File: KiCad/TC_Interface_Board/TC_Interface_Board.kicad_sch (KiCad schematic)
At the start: 23 parts, among them J1_24V_ROW1 Conn_01x04, J1_CN1_24V1 Conn_01x03, J2_CN2_9V_Main1 Conn_01x02, J3_CN3_9V_Main1 Conn_01x02, J4_BUS_MONITER1 Conn_01x05, Q1 DTC143E, Q2 DTC143E, U1 MC34063AP

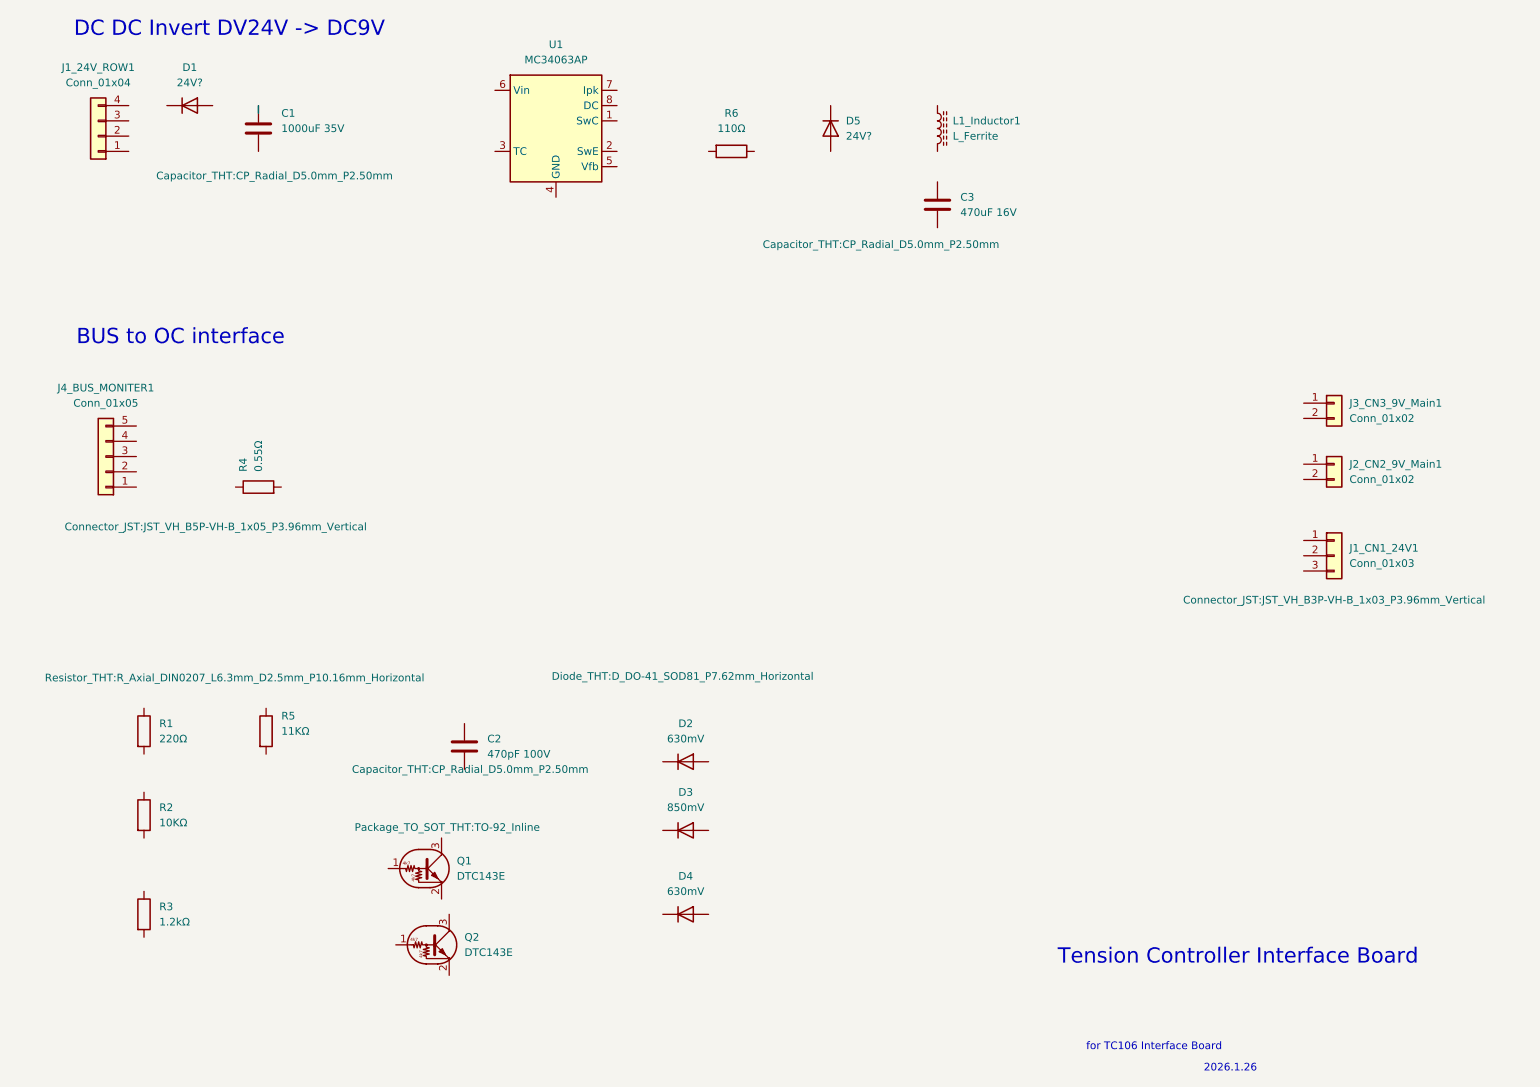
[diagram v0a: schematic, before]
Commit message: UPDATE
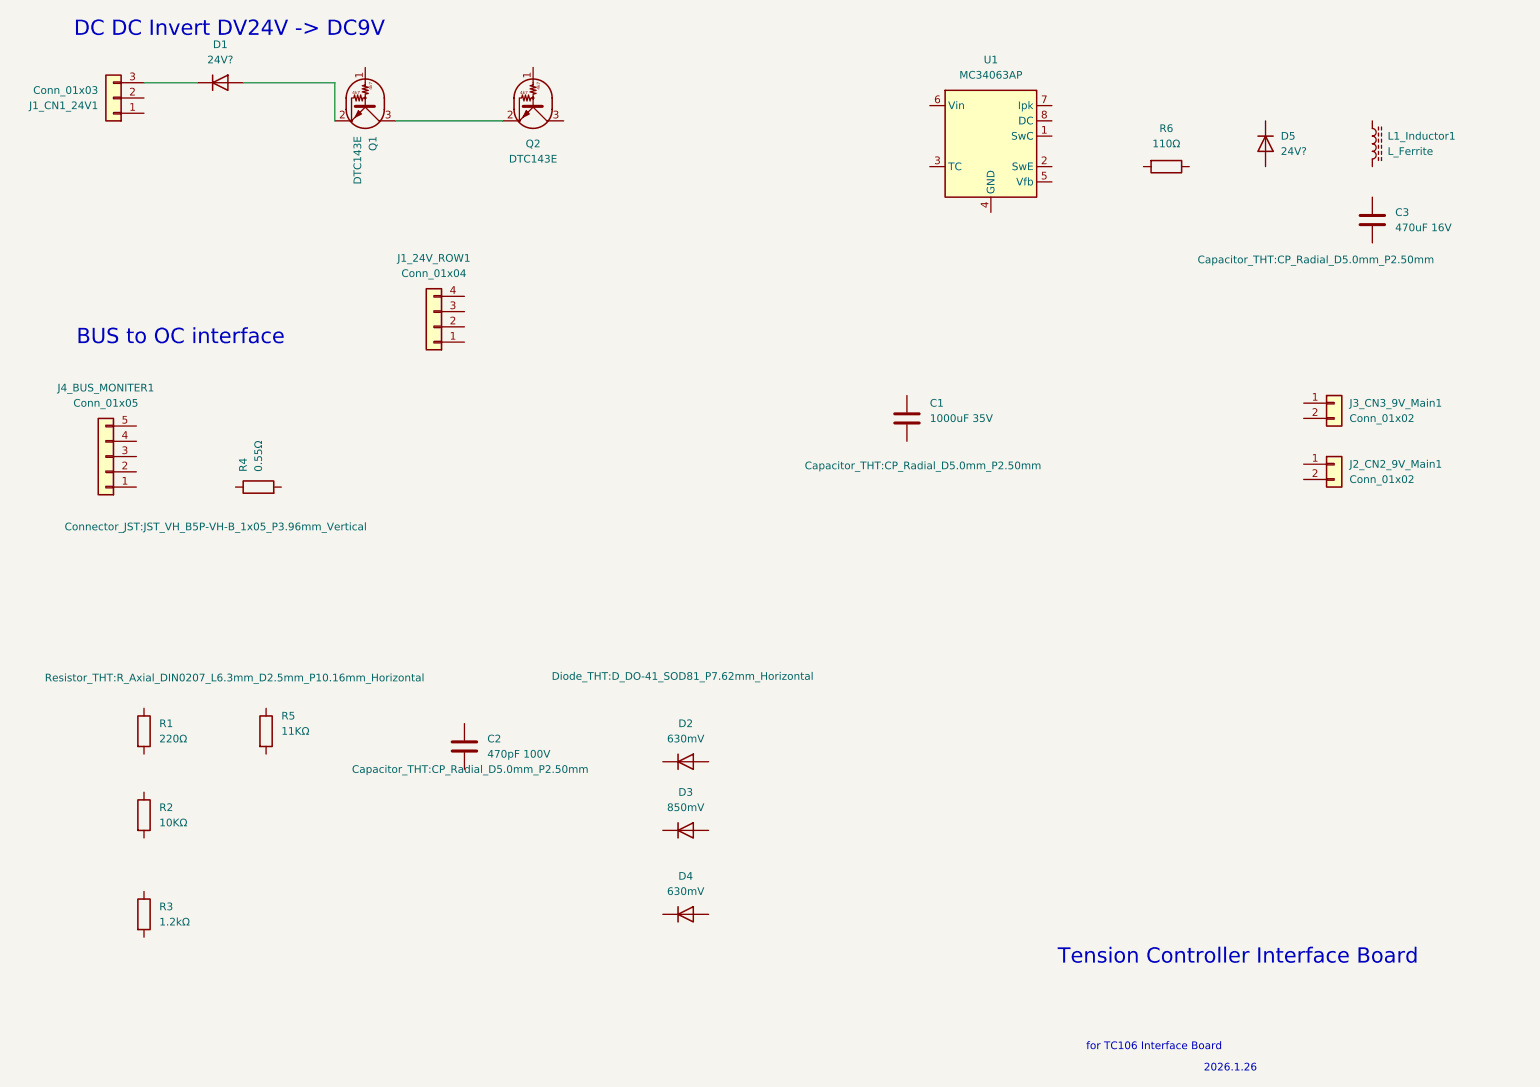
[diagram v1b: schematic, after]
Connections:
- net at Q2.2 (E): now also Q1.3 (C)
- net at D1.1 (K): now also J1_CN1_24V1.3 (Pin_3)
- net at D1.2 (A): now also Q1.2 (E)
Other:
- moved on the sheet: C1, C3, D1, D5, J1_24V_ROW1, J1_CN1_24V1, L1_Inductor1, Q1, Q2, R6, U1
